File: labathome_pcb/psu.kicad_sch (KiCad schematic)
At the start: 38 parts, among them J8 POWER, J9 Barrel_Jack_Switch, SW4 5V DIR, SW5 POWER, U11 AMS1117, U18 TPS2116DRL, U2 IP5306_I2C, U27 TPS54202DDC

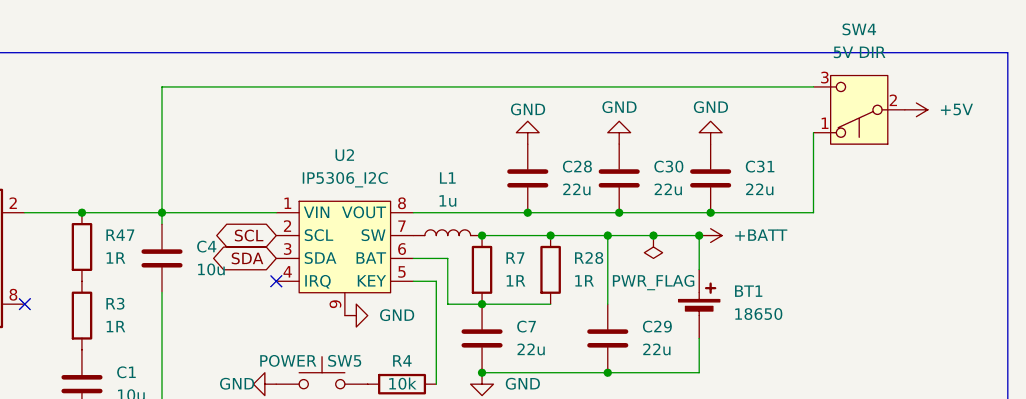
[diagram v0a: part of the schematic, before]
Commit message: Various
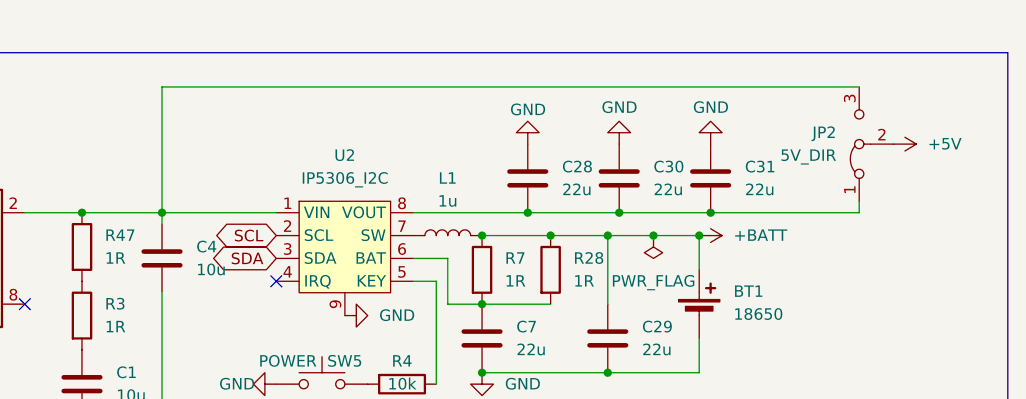
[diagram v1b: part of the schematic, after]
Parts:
- removed SW4: 5V DIR, liebler_MECH:Switch_SS12D00, symbol Switch:SW_Push_SPDT
- added JP2: 5V_DIR, Jumper:SolderJumper-3_P1.3mm_Bridged2Bar12_RoundedPad1.0x1.5mm, symbol Jumper:Jumper_3_Bridged12
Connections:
- net +5V: now also JP2.2 (C)
- net at C4.1, R47.1, U18.2 (VOUT)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: now also JP2.3 (B)
- net at C28.2, C30.2, C31.2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: now also JP2.1 (A)
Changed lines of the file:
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@@
 	(wire
 		(pts
-			(xy 219.71 33.02) (xy 231.14 33.02)
+			(xy 219.71 33.02) (xy 236.22 33.02)
 		)
 		(stroke
@@
 	(wire
 		(pts
-			(xy 231.14 19.05) (xy 158.75 19.05)
+			(xy 158.75 19.05) (xy 236.22 19.05)
 		)
 		(stroke
@@
 	(wire
 		(pts
-			(xy 231.14 33.02) (xy 231.14 24.13)
+			(xy 110.49 27.94) (xy 120.65 27.94)
 		)
 		(stroke
@@
 	(wire
 		(pts
-			(xy 110.49 27.94) (xy 120.65 27.94)
+			(xy 17.78 73.66) (xy 26.67 73.66)
 		)
 		(stroke
@@
 	(wire
 		(pts
-			(xy 17.78 73.66) (xy 26.67 73.66)
+			(xy 46.99 73.66) (xy 55.88 73.66)
 		)
 		(stroke
@@
 	(wire
 		(pts
-			(xy 46.99 73.66) (xy 55.88 73.66)
+			(xy 107.95 105.41) (xy 100.33 105.41)
 		)
 		(stroke
@@
 	(wire
 		(pts
-			(xy 107.95 105.41) (xy 100.33 105.41)
+			(xy 90.17 113.03) (xy 90.17 128.27)
 		)
 		(stroke
@@
 	(wire
 		(pts
-			(xy 90.17 113.03) (xy 90.17 128.27)
+			(xy 236.22 33.02) (xy 236.22 31.75)
 		)
 		(stroke
@@
 	)
 	(symbol
+		(lib_id "Jumper:Jumper_3_Bridged12")
+		(at 236.22 25.4 90)
+		(unit 1)
+		(exclude_from_sim yes)
+		(in_bom no)
+		(on_board yes)
+		(dnp no)
+		(fields_autoplaced yes)
+		(property "Reference" "JP2"
+			(at 233.68 24.1299 90)
+			(effects
+				(font
+					(size 1.27 1.27)
+				)
+				(justify left)
+			)
+		)
+		(property "Value" "5V_DIR"
+			(at 233.68 26.6699 90)
+			(effects
+				(font
+					(size 1.27 1.27)
+				)
+				(justify left)
+			)
+		)
+		(property "Footprint" "Jumper:SolderJumper-3_P1.3mm_Bridged2Bar12_RoundedPad1.0x1.5mm"
+			(at 236.22 25.4 0)
+			(effects
+				(font
+					(size 1.27 1.27)
+				)
+				(hide yes)
+			)
+		)
+		(property "Datasheet" "~"
+			(at 236.22 25.4 0)
+			(effects
+				(font
+					(size 1.27 1.27)
+				)
+				(hide yes)
+			)
+		)
+		(property "Description" "Jumper, 3-pole, pins 1+2 closed/bridged"
+			(at 236.22 25.4 0)
+			(effects
+				(font
+					(size 1.27 1.27)
+				)
+				(hide yes)
+			)
+		)
+		(pin "2"
+		)
+		(pin "3"
+		)
+		(pin "1"
+		)
+		(instances
+			(project ""
+				(path "/e4d6926a-1a8b-424d-97c4-66b6ad87e4ac/77dfbe0c-d674-478a-bf0e-cfa040fb2e8f"
+					(reference "JP2")
+					(unit 1)
+				)
+			)
+		)
+	)
+	(symbol
 		(lib_id "liebler_SEMICONDUCTORS:IP5306_I2C")
 		(at 179.07 36.83 0)
@@
 	)
 	(symbol
-		(lib_id "Switch:SW_Push_SPDT")
-		(at 236.22 21.59 180)
-		(unit 1)
-		(exclude_from_sim no)
-		(in_bom yes)
-		(on_board yes)
-		(dnp no)
-		(fields_autoplaced yes)
-		(property "Reference" "SW4"
-			(at 236.22 12.7 0)
-			(effects
-				(font
-					(size 1.27 1.27)
-				)
-			)
-		)
-		(property "Value" "5V DIR"
-			(at 236.22 15.24 0)
-			(effects
-				(font
-					(size 1.27 1.27)
-				)
-			)
-		)
-		(property "Footprint" "liebler_MECH:Switch_SS12D00"
-			(at 236.22 21.59 0)
-			(effects
-				(font
-					(size 1.27 1.27)
-				)
-				(hide yes)
-			)
-		)
-		(property "Datasheet" "~"
-			(at 236.22 21.59 0)
-			(effects
-				(font
-					(size 1.27 1.27)
-				)
-				(hide yes)
-			)
-		)
-		(property "Description" "Momentary Switch, single pole double throw"
-			(at 236.22 21.59 0)
-			(effects
-				(font
-					(size 1.27 1.27)
-				)
-				(hide yes)
-			)
-		)
-		(pin "3"
-		)
-		(pin "2"
-		)
-		(pin "1"
-		)
-		(instances
-			(project ""
-				(path "/e4d6926a-1a8b-424d-97c4-66b6ad87e4ac/77dfbe0c-d674-478a-bf0e-cfa040fb2e8f"
-					(reference "SW4")
-					(unit 1)
-				)
-			)
-		)
-	)
-	(symbol
 		(lib_id "Device:C")
 		(at 20.32 113.03 180)
@@
 	(symbol
 		(lib_id "power:+5V")
-		(at 241.3 21.59 270)
+		(at 240.03 25.4 270)
 		(unit 1)
 		(exclude_from_sim no)
@@
 		(fields_autoplaced yes)
 		(property "Reference" "#PWR037"
-			(at 237.49 21.59 0)
+			(at 236.22 25.4 0)
 			(effects
 				(font
@@
 		)
 		(property "Value" "+5V"
-			(at 245.11 21.5899 90)
+			(at 243.84 25.3999 90)
 			(effects
 				(font
@@
 		)
 		(property "Footprint" ""
-			(at 241.3 21.59 0)
+			(at 240.03 25.4 0)
 			(effects
 				(font
@@
 		)
 		(property "Datasheet" ""
-			(at 241.3 21.59 0)
+			(at 240.03 25.4 0)
 			(effects
 				(font
@@
 		)
 		(property "Description" "Power symbol creates a global label with name \"+5V\""
-			(at 241.3 21.59 0)
+			(at 240.03 25.4 0)
 			(effects
 				(font

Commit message: Minor improments on pcb
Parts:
- J8: footprint liebler_CONN:USB_C_Receptacle_HRO_TYPE-C-31-M-12_IMPROVED -> liebler_CONN:USB_C_Receptacle_HRO_TYPE-C-31-M-12_smaller
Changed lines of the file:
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@@
 			)
 		)
-		(property "Footprint" "liebler_CONN:USB_C_Receptacle_HRO_TYPE-C-31-M-12_IMPROVED"
+		(property "Footprint" "liebler_CONN:USB_C_Receptacle_HRO_TYPE-C-31-M-12_smaller"
 			(at 29.21 36.83 0)
 			(effects
